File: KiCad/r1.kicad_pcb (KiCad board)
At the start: 2 copper layers, 215.9 x 127 mm, 75 parts, among them J1 KEYBOARD, J3 ATX-20, J4 DE9_Socket, J5 R1 EXPANSION, Q1 2N4401, U1 6502, U10 74LS245, U11 MAX232, U2 6821, U3 27C64, U4 HM62256BLP, U5 74LS138, U6 74LS00, U7 74LS04, U8 P8X32A-D40, U9 24LC256, X1 1 MHz, X2 5MHz

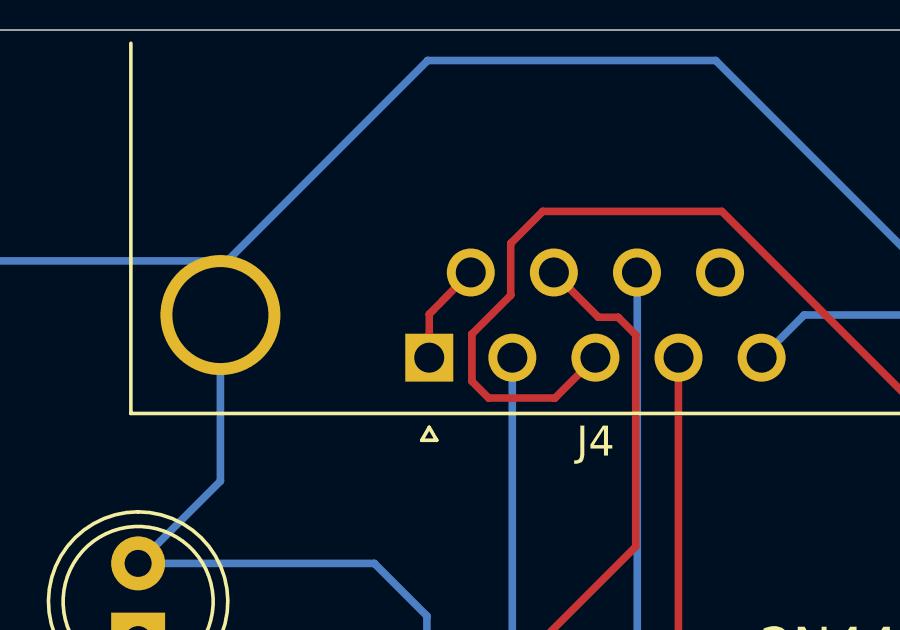
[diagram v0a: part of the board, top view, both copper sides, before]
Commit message: R20260909
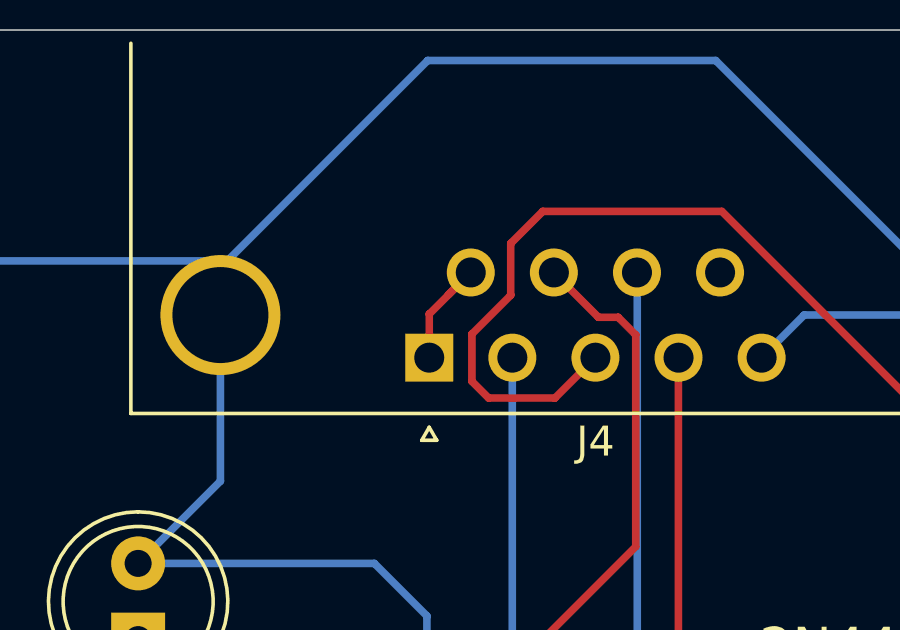
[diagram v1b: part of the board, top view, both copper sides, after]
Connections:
- R19 pad 1: unconnected-(R19-Pad1) -> /KCL
- R19 pad 2: unconnected-(R19-Pad2) -> Net-(J6-Pad5)
- R20 pad 1: Net-(D1-K) -> Net-(J6-Pad1)
- R20 pad 2: /VCC -> /DATA
- R22 pad 1: unconnected-(R22-Pad1) -> /VCC
- R22 pad 2: unconnected-(R22-Pad2) -> Net-(D1-K)
- R25 pad 1: Net-(C13-Pad2) -> Net-(Q1-B)
- R25 pad 2: Net-(Q1-B) -> Net-(C13-Pad2)
- R7 pad 1: unconnected-(R7-Pad1) -> /VDD
- R7 pad 2: unconnected-(R7-Pad2) -> Net-(J6-Pad5)
- R8 pad 1: unconnected-(R8-Pad1) -> /VDD
- R8 pad 2: unconnected-(R8-Pad2) -> Net-(J6-Pad1)
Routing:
- net (no net): track 10338.8 -> 9718.6 mm
- net /A2: track 0.00 -> 238.4 mm
- net GND: track 518.5 -> 653.0 mm
- net /VCC: track 562.3 -> 682.5 mm
- net /VDD: track 240.8 -> 346.7 mm
- net unconnected-(R22-Pad2): track 60.0 -> 0.00 mm, vias 1 -> 0
- net Net-(D1-K): track 0.00 -> 60.0 mm, vias 0 -> 1
- net Net-(Q1-B): track 0.00 -> 16.1 mm
- net unconnected-(R7-Pad2): track 15.0 -> 0.00 mm, vias 1 -> 0
- net Net-(J6-Pad5): track 0.00 -> 15.0 mm, vias 0 -> 1
- net Net-(C13-Pad2): track 0.00 -> 4.86 mm
- net Net-(J4-Pad1): track 3.41 -> 4.46 mm
